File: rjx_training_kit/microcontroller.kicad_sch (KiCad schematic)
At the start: 7 parts, among them SW2 SW_Push, U1 STM32F407VGTx

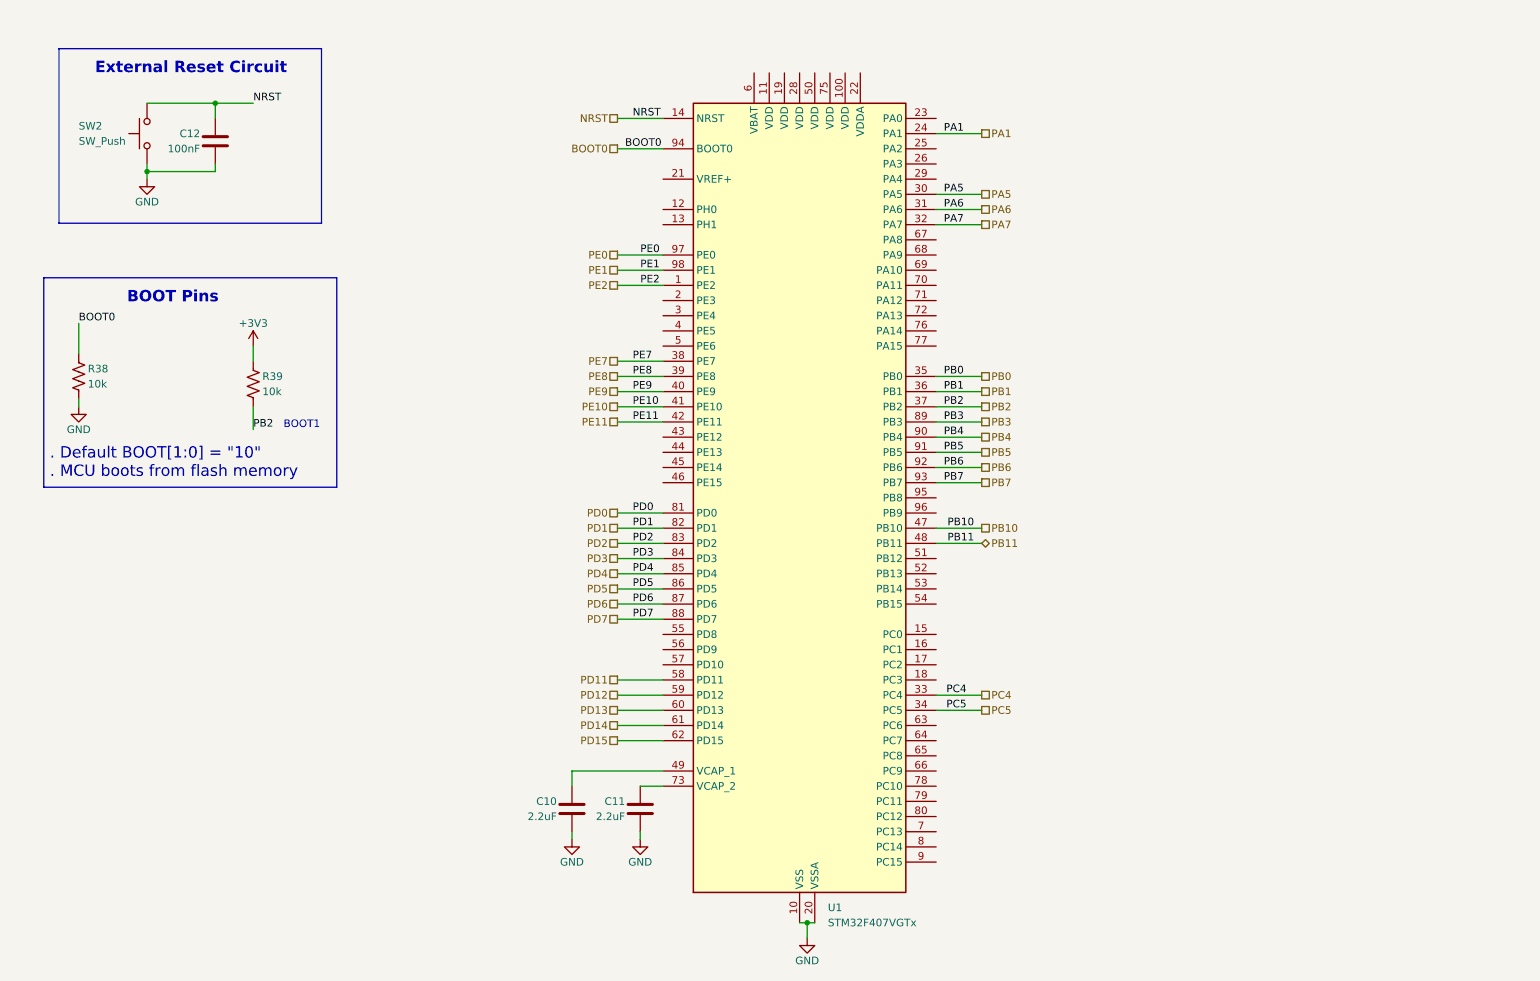
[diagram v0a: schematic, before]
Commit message: Update
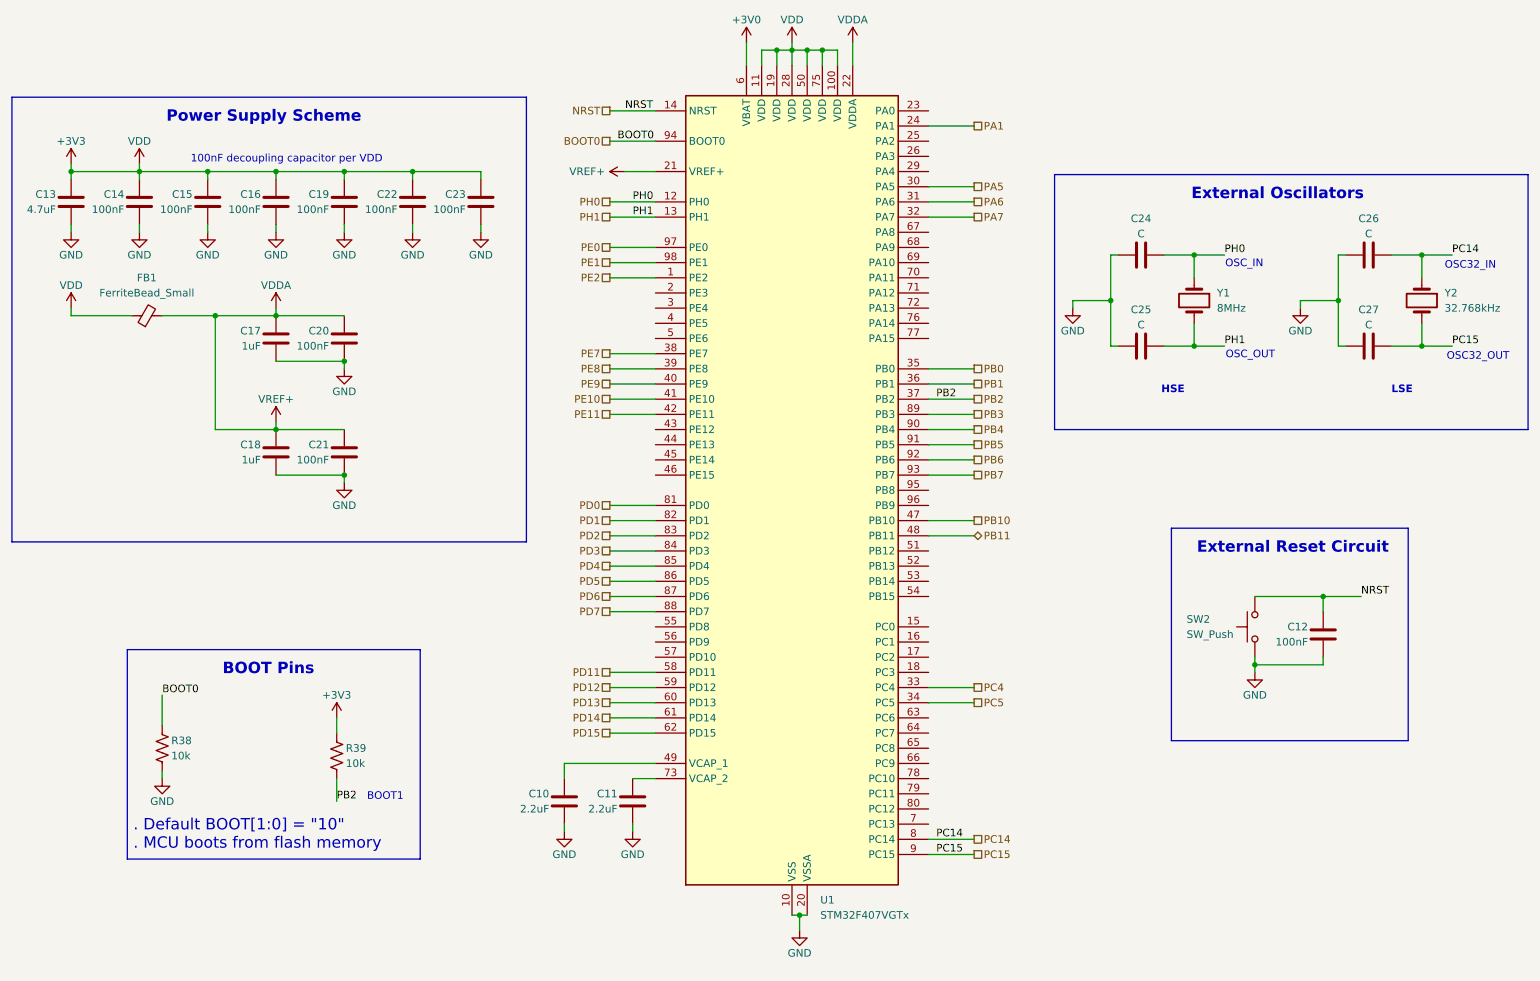
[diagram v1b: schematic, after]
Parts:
- added C13: 4.7uF, symbol Device:C
- added C14, C15, C16, C19, C20, C21, C22, C23: 100nF, symbol Device:C
- added C17, C18: 1uF, symbol Device:C
- added C24, C25, C26, C27: C, symbol Device:C
- added FB1: FerriteBead_Small, symbol Device:FerriteBead_Small
- added Y1: 8MHz, symbol Device:Crystal
- added Y2: 32.768kHz, symbol Device:Crystal
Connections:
- net +3V3: now also U1.100 (VDD), U1.11 (VDD), U1.19 (VDD), U1.28 (VDD), U1.50 (VDD), U1.75 (VDD), C13.1, C14.1, C15.1, C16.1, C19.1, C22.1, C23.1, FB1.1
- net GND: now also C13.2, C14.2, C15.2, C16.2, C17.2, C18.2, C19.2, C20.2, C21.2, C22.2, C23.2, C24.1, C25.1, C26.1, C27.1
- net PH0: now reaches U1.12 (PH0)
- net PH0: now also C24.2, Y1.1
- net PH1: now reaches U1.13 (PH1)
- net PH1: now also C25.2, Y1.2
- net VDDA: now reaches U1.21 (VREF+)
- net VDDA: now also U1.22 (VDDA), C17.1, C18.1, C20.1, C21.1, FB1.2
- net +3V0: now reaches U1.6 (VBAT)
- net PC14: now reaches U1.8 (PC14)
- net PC14: now also C26.2, Y2.1
- net PC15: now reaches U1.9 (PC15)
- net PC15: now also C27.2, Y2.2
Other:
- note added: "100nF decoupling capacitor per VDD"
- note added: "External Oscillators"
- note added: "HSE"
- note added: "LSE"
- note added: "OSC32_IN"
- note added: "OSC32_OUT"
- note added: "OSC_IN"
- note added: "OSC_OUT"
- note added: "Power Supply Scheme"
- moved on the sheet: C10, C11, C12, R38, R39, SW2, U1
